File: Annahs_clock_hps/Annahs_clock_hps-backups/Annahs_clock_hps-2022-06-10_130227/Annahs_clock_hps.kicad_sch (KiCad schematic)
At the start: 39 parts, among them J1 Conn_01x06, J2 Power_inlet_vertical, SW1 Omron_B3F_SPST, SW2 Omron_B3F_SPST, SW3 Omron_B3F_SPST, SW4 Omron_B3F_SPST, SW5 Omron_B3F_SPST, U1 DS1307_DIP-8, U2 MAX7219, U3 L7805, U4 SC56-11EWA, U5 SC56-11EWA, Y1 Crystal_16MHz

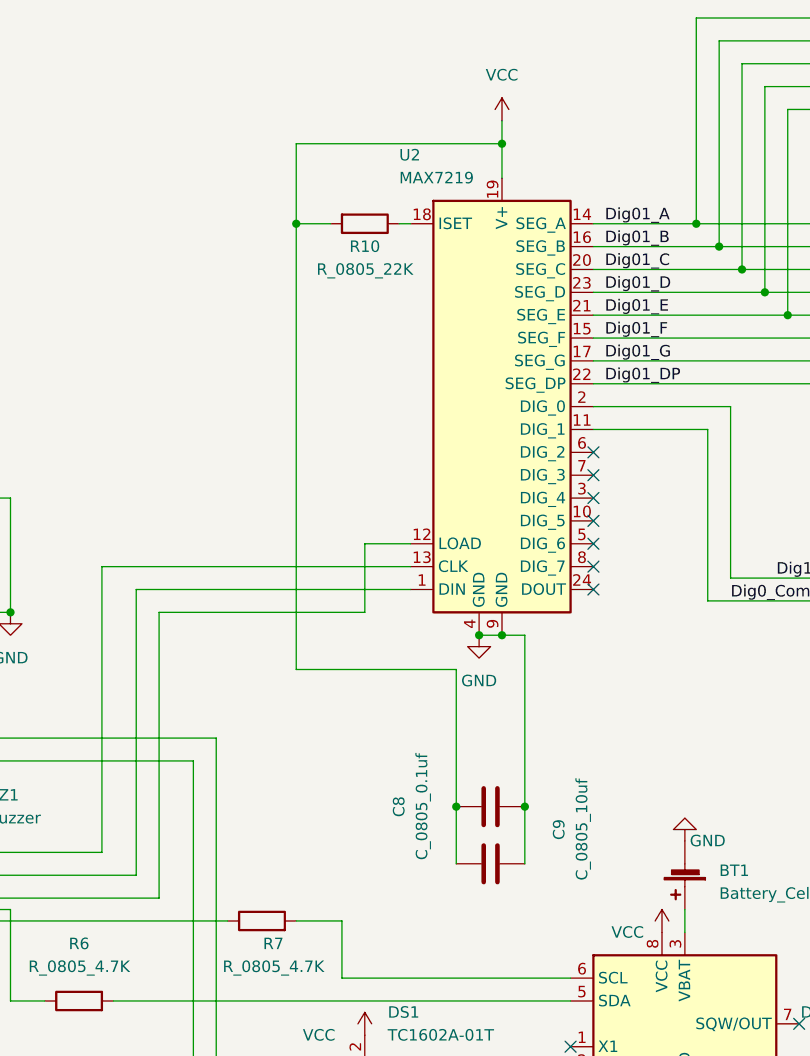
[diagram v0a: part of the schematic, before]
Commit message: Displays_firmware
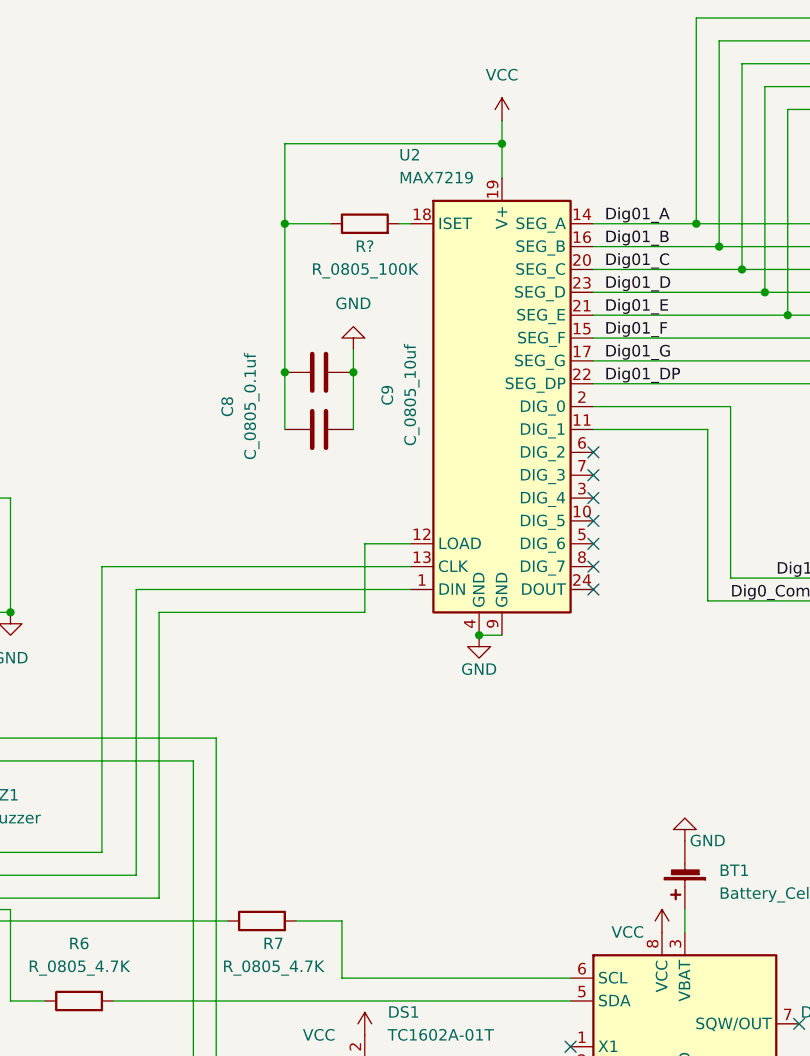
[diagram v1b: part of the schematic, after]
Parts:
- removed R10: R_0805_22K, footprints:R_0805_2012Metric, symbol HPS:R_0805_22K
- added R?: R_0805_100K, footprints:R_0805_2012Metric, symbol HPS:R_0805_100K
- U3: footprint (none) -> footprints:TO-220-3_Vertical
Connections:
- net VCC: now also R?.1
- net at U2.18 (ISET): now also R?.2
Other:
- moved on the sheet: C8, C9
